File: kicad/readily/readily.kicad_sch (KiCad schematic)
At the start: 29 parts, among them J1 Conn_01x09_Socket, J2 Micro_SD_Card_Det1, J3 USB_C_Receptacle_USB2.0_16P, J4 Conn_01x03, SW2 SW_SPST, SW3 SW_SPST, U1 ESP32-S3-WROOM-1, U2 BQ24040DSQR, U3 TPD2EUSB30, U4 TLV75533PDRV

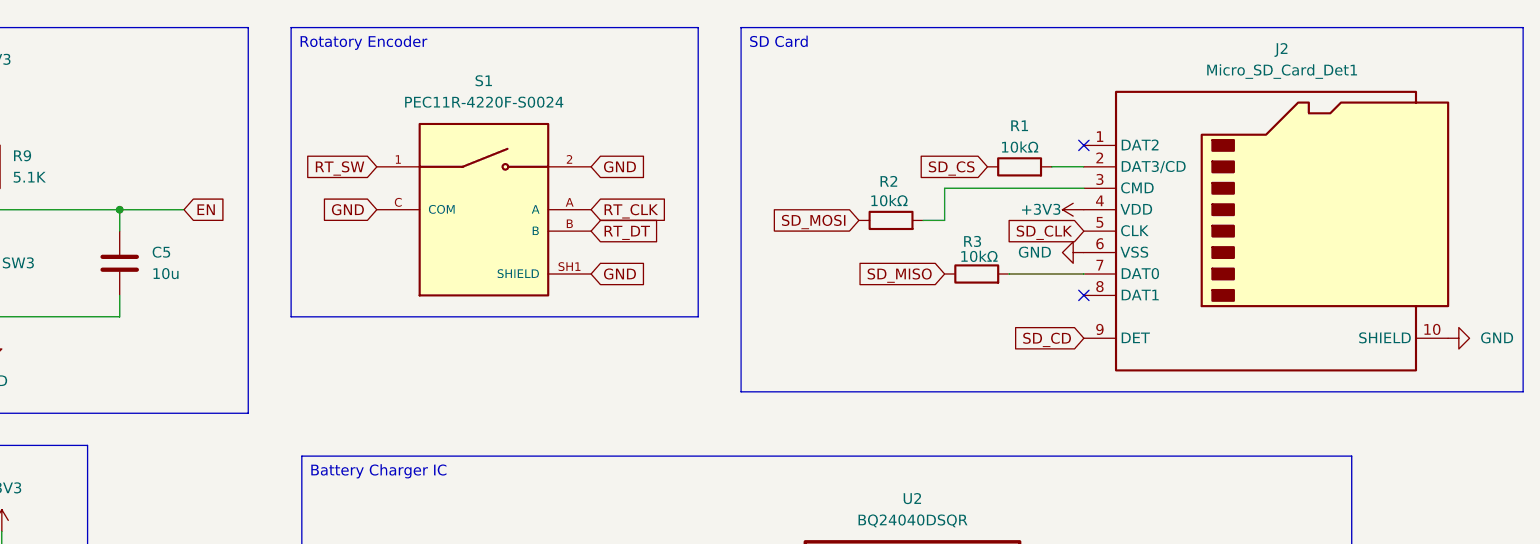
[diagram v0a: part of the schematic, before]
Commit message: feat: adding the first stage of the PCB
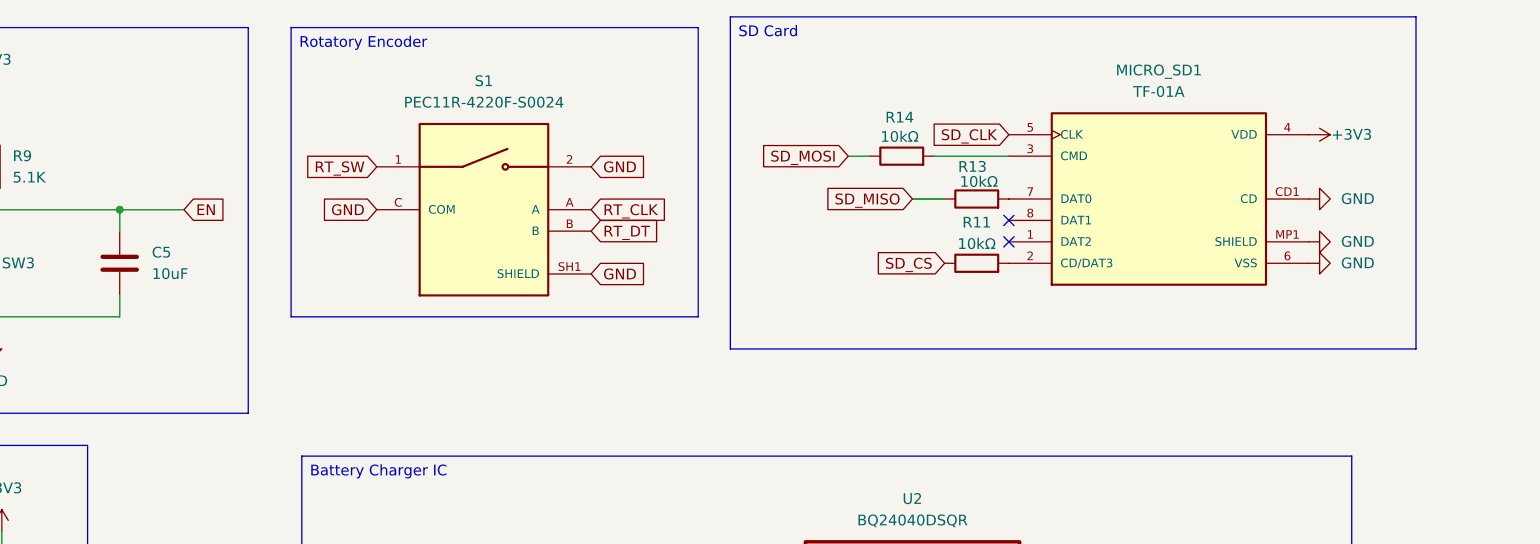
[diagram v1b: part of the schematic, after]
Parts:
- removed J2: Micro_SD_Card_Det1, symbol Connector:Micro_SD_Card_Det1
- removed R1, R2, R3: 10kΩ, symbol Device:R
- added MICRO_SD1: TF-01A, TF-01A:TF-01A, symbol TF-01A:TF-01A
- added R11, R13, R14: 10kΩ, PCM_JLCPCB:R_0603, symbol Device:R
- C1: footprint (none) -> PCM_JLCPCB:C_0603
- C2, C3: footprint (none) -> PCM_JLCPCB:C_0805
- C4: footprint Capacitor_SMD:C_0402_1005Metric -> PCM_JLCPCB:C_0603
- C5: value 10u -> 10uF; footprint Capacitor_SMD:C_0805_2012Metric -> PCM_JLCPCB:C_0805
- J1: footprint (none) -> Pin01x09:Pins01x09
- J3: footprint (none) -> Connector_USB:USB_C_Receptacle_HRO_TYPE-C-31-M-12
- J4: footprint (none) -> JST_PH_B3B-PH-K_1x03_P2.00mm_Vertical
- R10, R12, R9: footprint Resistor_SMD:R_0402_1005Metric -> PCM_JLCPCB:R_0603
- R4, R5, R6, R7, R8: footprint (none) -> PCM_JLCPCB:R_0603
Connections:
- net +3V3: now also MICRO_SD1.4 (VDD)
- net GND: now also MICRO_SD1.6 (VSS), MICRO_SD1.CD1 (CD), MICRO_SD1.MP1 (SHIELD), MICRO_SD1.MP2 (SHIELD), MICRO_SD1.MP3 (SHIELD), MICRO_SD1.MP4 (SHIELD)
- net SD_CLK: now also MICRO_SD1.5 (CLK)
- net SD_CS: now also R11.1
- net SD_MISO: now also R13.1
- net SD_MOSI: now also R14.1
- new net: MICRO_SD1.7 (DAT0), R13.2
- new net: MICRO_SD1.2 (CD/DAT3), R11.2
- new net: MICRO_SD1.3 (CMD), R14.2
